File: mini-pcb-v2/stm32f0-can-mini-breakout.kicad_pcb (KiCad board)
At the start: 2 copper layers, 91.4 x 53.7 mm, 108 parts, among them J1 POWER_BUS, J10 I2C, J11 GS2, J12 Conn_01x02, J13 Conn_01x09, J14 Conn_01x09, J15 Conn_01x09, J16 Conn_01x09, J17 Conn_01x09, J18 Conn_01x09, J19 Conn_01x08, J2 POWER_BUS, J20 Conn_01x08, J21 Conn_01x08, J22 Conn_01x05, J23 Conn_01x05, J25 Conn_01x05, J26 Conn_01x04, J27 Conn_01x09, J28 Conn_01x04, J29 Conn_01x02, J3 GS2, J30 Conn_01x04, J31 Conn_01x02, J32 Conn_01x02, J33 Conn_01x04, J34 Conn_01x02, J35 Conn_01x04, J36 USB, J37 Conn_01x09, J38 Conn_01x09, J4 GS2, J41 Conn_01x02, J46 Screw_Terminal_01x02, J47 Screw_Terminal_01x02, J48 Screw_Terminal_01x02, J49 Screw_Terminal_01x02, J5 GS2, J6 UART, J7 SWD, J8 STEPDOWN, J9 I2C, Q1 N-FET, Q10 BT138-800, Q11 BT138-800, Q12 BT138-800, Q2 N-FET, Q3 N-FET, Q9 BT138-800, U1 AT24CS64-SSHM, U2 SN65HVD230, U3 STM32F072C8Tx, U4 MOC3063M, U5 MOC3063M, U6 MOC3063M, U7 MOC3063M, Y1 Crystal

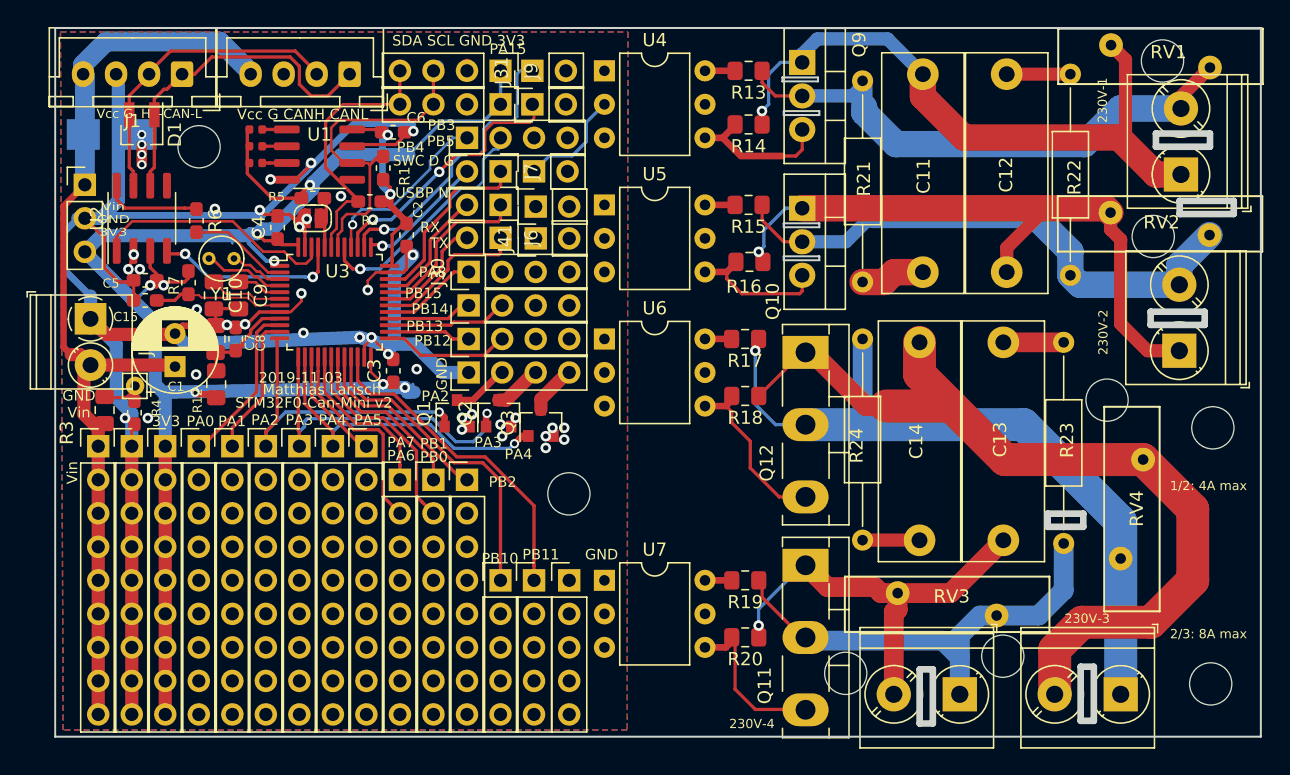
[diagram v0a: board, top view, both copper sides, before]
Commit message: update v2pcb
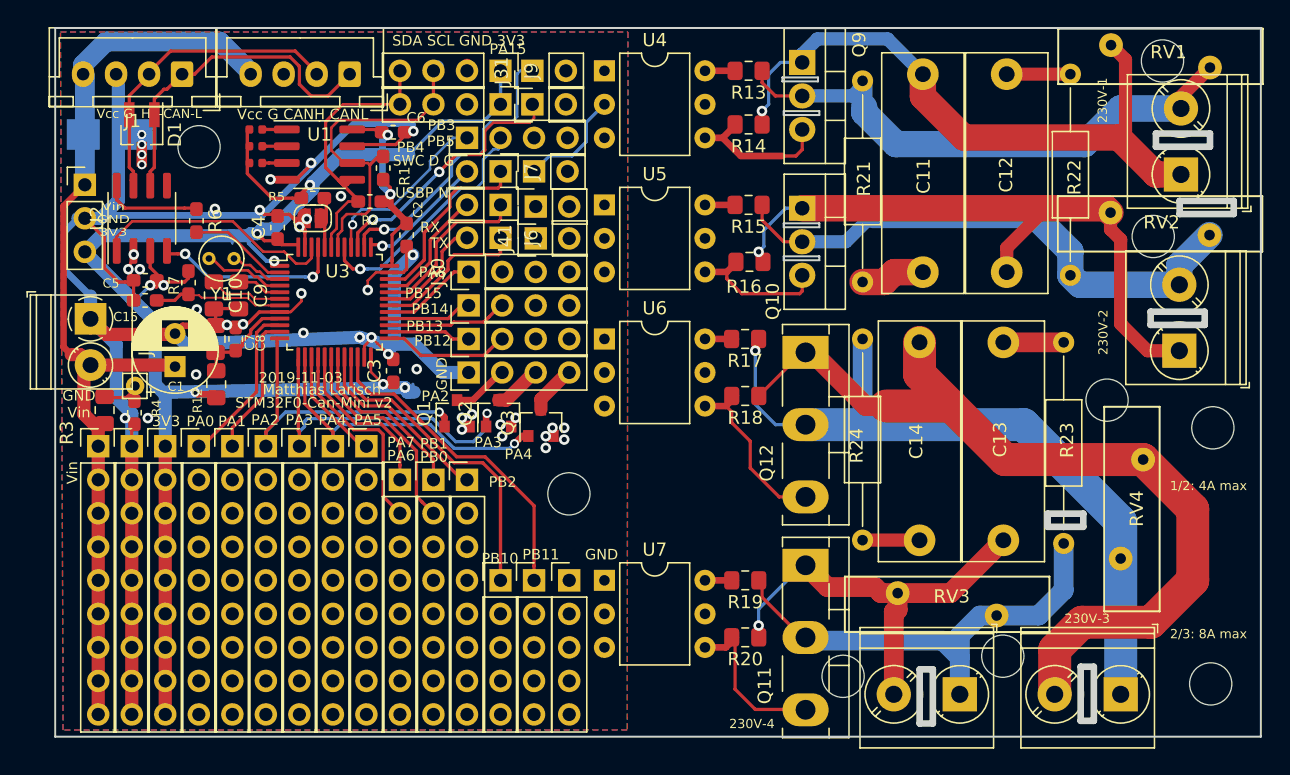
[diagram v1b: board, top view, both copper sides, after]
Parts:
- moved REF** 0.30 mm to (120.7, 71.0)
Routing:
- net SDA: track 20.6 -> 21.9 mm
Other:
- net class Default: clearance 0.18 -> 0.17
- rule trace_clearance: 0.18 -> 0.17
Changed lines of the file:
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@@
     (thickness 1.6)
     (drawings 95)
-    (tracks 850)
+    (tracks 856)
     (zones 0)
     (modules 108)
@@
   )
   (setup
-    (last_trace_width 1.5)
+    (last_trace_width 0.25)
     (user_trace_width 0.15)
     (user_trace_width 0.2)
@@
     (user_trace_width 2)
     (user_trace_width 2.5)
-    (trace_clearance 0.18)
+    (trace_clearance 0.17)
     (zone_clearance 0.508)
     (zone_45_only no)
@@
     (visible_elements FFFFFF7F)
     (pcbplotparams
-      (layerselection 0x010f0_80000001)
+      (layerselection 0x010f0_ffffffff)
       (usegerberextensions false)
-      (usegerberattributes false)
+      (usegerberattributes true)
       (usegerberadvancedattributes false)
       (creategerberjobfile false)
@@
   (net 73 "Net-(C15-Pad2)")
   (net_class Default "Dies ist die voreingestellte Netzklasse."
-    (clearance 0.18)
+    (clearance 0.17)
     (trace_width 0.25)
     (via_dia 0.6)
@@
   )
   (module MountingHole:MountingHole_3.2mm_M3 (layer F.Cu)
-    (at 120.9 70.8)
+    (at 120.7 71.025)
     (descr "Mounting Hole 3.2mm, no annular, M3")
     (tags "mounting hole 3.2mm no annular m3")
@@
   (via (at 68.0212 51.4604) (size 0.8) (drill 0.4) (layers F.Cu B.Cu) (net 2))
   (via (at 71.7296 43.2308) (size 0.8) (drill 0.4) (layers F.Cu B.Cu) (net 2))
-  (via (at 75.3872 44.3484) (size 0.8) (drill 0.4) (layers F.Cu B.Cu) (net 2))
+  (via (at 75.2348 44.3484) (size 0.8) (drill 0.4) (layers F.Cu B.Cu) (net 2))
   (via (at 74.0156 44.3992) (size 0.8) (drill 0.4) (layers F.Cu B.Cu) (net 2))
   (via (at 71.6788 48.1584) (size 0.8) (drill 0.4) (layers F.Cu B.Cu) (net 2))
@@
   (segment (start 82.737209 36.361868) (end 83.097076 36.002001) (width 0.2) (layer F.Cu) (net 14))
   (segment (start 87.122 27.686) (end 86.521495 27.686) (width 0.2) (layer F.Cu) (net 15))
-  (segment (start 83.632 35.052) (end 83.082 35.052) (width 0.2) (layer F.Cu) (net 15))
-  (segment (start 81.919 37.499977) (end 81.919 38.322) (width 0.2) (layer F.Cu) (net 15))
-  (segment (start 83.082 35.052) (end 82.329001 35.804999) (width 0.2) (layer F.Cu) (net 15))
-  (segment (start 82.329001 35.804999) (end 82.329001 37.089976) (width 0.2) (layer F.Cu) (net 15))
-  (segment (start 82.329001 37.089976) (end 81.919 37.499977) (width 0.2) (layer F.Cu) (net 15))
   (segment (start 87.122 25.146) (end 87.122 27.686) (width 0.25) (layer F.Cu) (net 15))
   (segment (start 85.919919 27.686) (end 87.122 27.686) (width 0.2) (layer F.Cu) (net 15))
@@
   (segment (start 81.91135 28.57865) (end 82.804 27.686) (width 0.2) (layer F.Cu) (net 15))
   (segment (start 81.91135 28.57865) (end 81.489989 29.000011) (width 0.25) (layer F.Cu) (net 15))
-  (segment (start 81.489989 32.467989) (end 83.726 34.704) (width 0.25) (layer F.Cu) (net 15))
   (segment (start 81.489989 29.000011) (end 81.489989 32.467989) (width 0.25) (layer F.Cu) (net 15))
   (segment (start 83.726 34.704) (end 83.726 34.958) (width 0.25) (layer F.Cu) (net 15))
   (segment (start 83.726 34.958) (end 83.632 35.052) (width 0.25) (layer F.Cu) (net 15))
+  (segment (start 82.79371 33.77171) (end 82.4738 33.4518) (width 0.25) (layer F.Cu) (net 15))
+  (segment (start 83.501 33.401) (end 83.13029 33.77171) (width 0.25) (layer F.Cu) (net 15))
+  (segment (start 83.13029 33.77171) (end 82.79371 33.77171) (width 0.25) (layer F.Cu) (net 15))
+  (segment (start 81.489989 32.467989) (end 82.4738 33.4518) (width 0.25) (layer F.Cu) (net 15))
+  (segment (start 82.4738 33.4518) (end 83.726 34.704) (width 0.25) (layer F.Cu) (net 15))
+  (segment (start 81.919 37.499977) (end 81.919 38.322) (width 0.2) (layer F.Cu) (net 15))
+  (segment (start 82.329001 37.089976) (end 81.919 37.499977) (width 0.2) (layer F.Cu) (net 15))
+  (segment (start 82.329001 35.933399) (end 82.329001 37.089976) (width 0.2) (layer F.Cu) (net 15))
+  (segment (start 83.632 35.052) (end 83.2104 35.052) (width 0.2) (layer F.Cu) (net 15))
+  (segment (start 83.2104 35.052) (end 82.329001 35.933399) (width 0.2) (layer F.Cu) (net 15))
   (segment (start 81.544 36.322) (end 81.544 34.874) (width 0.25) (layer F.Cu) (net 16))
   (segment (start 81.544 34.874) (end 81.468 34.798) (width 0.25) (layer F.Cu) (net 16))
@@
   (segment (start 94.214398 31.0896) (end 94.5896 31.0896) (width 0.2) (layer B.Cu) (net 72))
   (segment (start 93.4212 31.882798) (end 94.214398 31.0896) (width 0.2) (layer B.Cu) (net 72))
-  (segment (start 71.9 42.15) (end 71.1 42.15) (width 0.15) (layer F.Cu) (net 73))
   (segment (start 69.318 42.545) (end 68.693 42.545) (width 0.25) (layer F.Cu) (net 73))
   (segment (start 70.525 42.075) (end 70.055 42.545) (width 0.25) (layer F.Cu) (net 73))
   (segment (start 70.055 42.545) (end 69.318 42.545) (width 0.25) (layer F.Cu) (net 73))
   (segment (start 71.1 42.075) (end 70.525 42.075) (width 0.25) (layer F.Cu) (net 73))
-  (segment (start 76.18848 42.922) (end 78.0065 42.922) (width 0.15) (layer F.Cu) (net 73))
-  (segment (start 76.18448 42.926) (end 76.18848 42.922) (width 0.15) (layer F.Cu) (net 73))
-  (segment (start 72.08899 42.33899) (end 75.59747 42.33899) (width 0.15) (layer F.Cu) (net 73))
   (segment (start 71.9 42.15) (end 72.08899 42.33899) (width 0.15) (layer F.Cu) (net 73))
-  (segment (start 75.59747 42.33899) (end 76.18448 42.926) (width 0.15) (layer F.Cu) (net 73))
+  (segment (start 73.772427 42.33899) (end 73.792428 42.358991) (width 0.15) (layer F.Cu) (net 73))
+  (segment (start 73.792428 42.358991) (end 75.589187 42.358991) (width 0.15) (layer F.Cu) (net 73))
+  (segment (start 77.169 42.922) (end 78.0065 42.922) (width 0.15) (layer F.Cu) (net 73))
+  (segment (start 76.152196 42.922) (end 77.169 42.922) (width 0.15) (layer F.Cu) (net 73))
+  (segment (start 75.589187 42.358991) (end 76.152196 42.922) (width 0.15) (layer F.Cu) (net 73))
+  (segment (start 71.1 42.15) (end 71.9 42.15) (width 0.15) (layer F.Cu) (net 73))
+  (segment (start 72.08899 42.33899) (end 73.772427 42.33899) (width 0.15) (layer F.Cu) (net 73))
   (zone (net 2) (net_name GND) (layer B.Cu) (hatch edge 0.508)
     (connect_pads (clearance 0.35))
